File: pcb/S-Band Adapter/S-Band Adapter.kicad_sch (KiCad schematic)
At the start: 5 parts, among them J1 CT3151SP-2, J2 FTSH-107-01-L-DV-K-A, J3 ERF8-030-05.0-L-DV-TR, J4 532611071

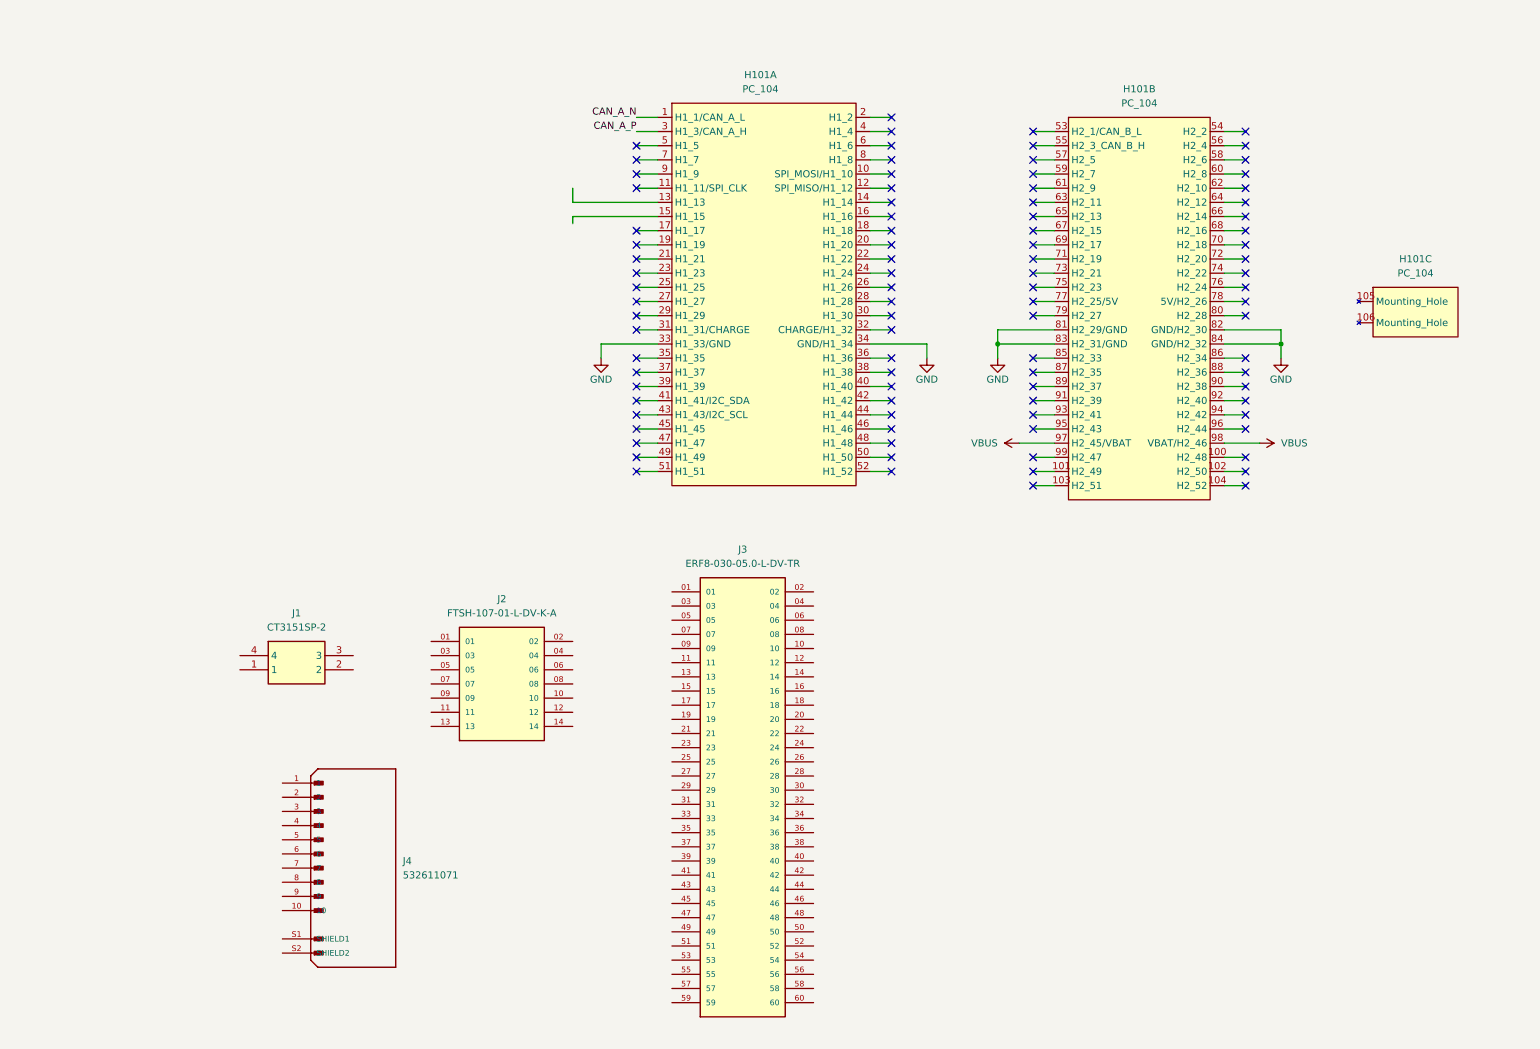
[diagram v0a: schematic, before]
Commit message: Finished PCB
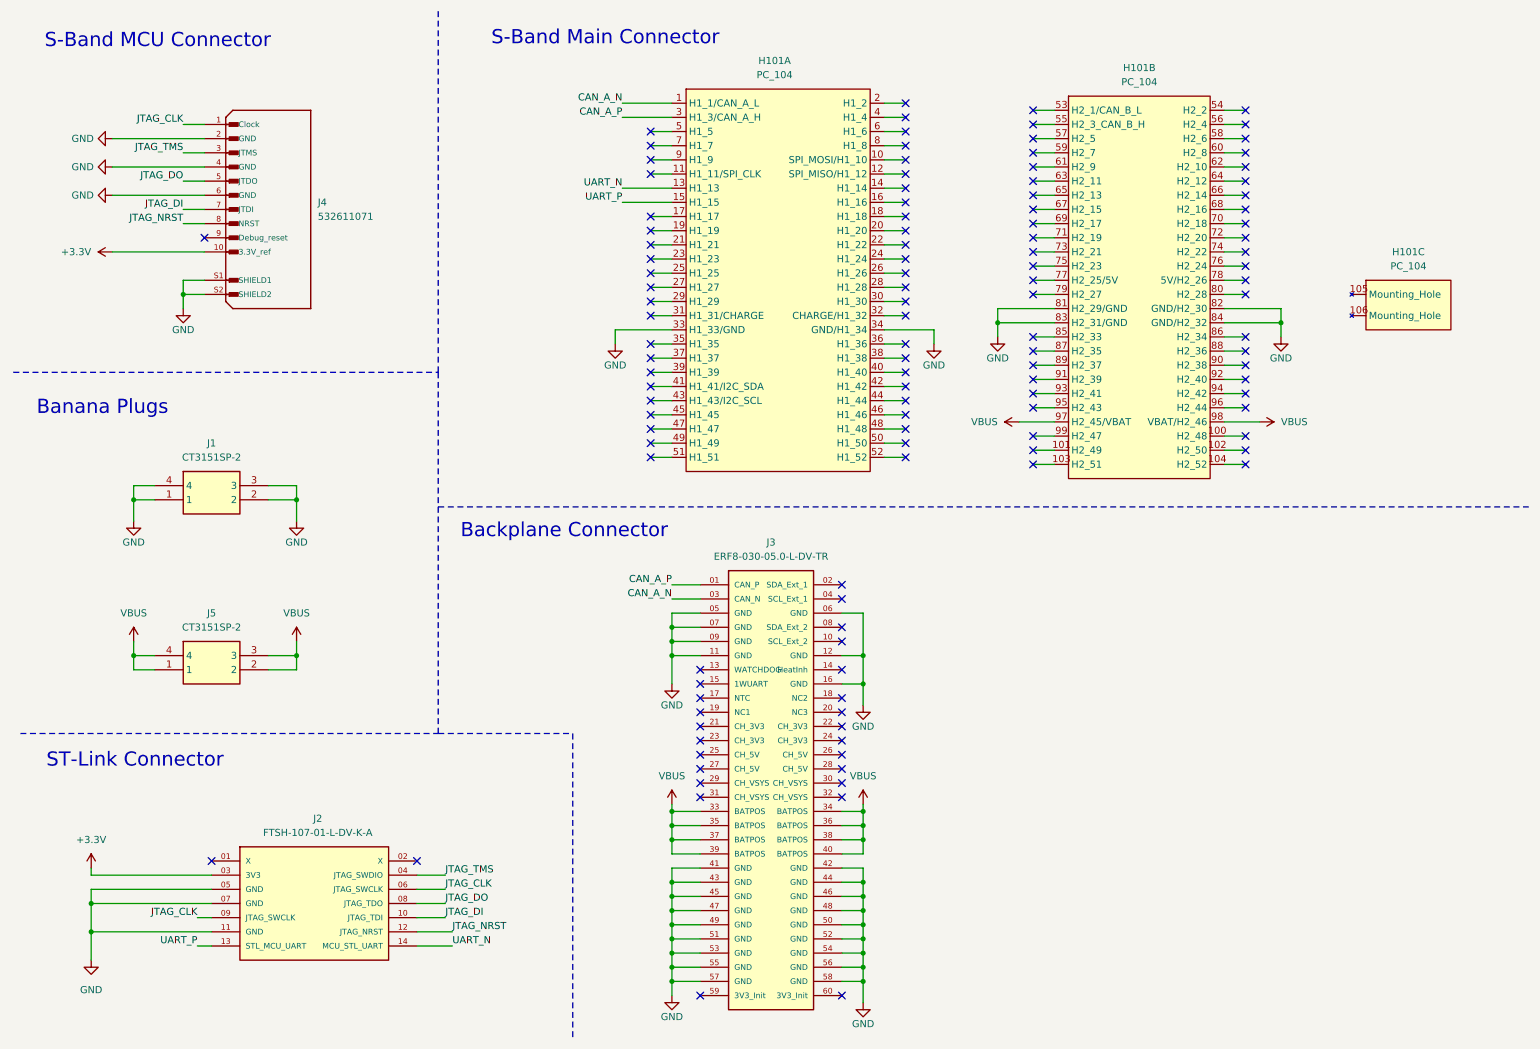
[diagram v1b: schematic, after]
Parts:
- added J5: CT3151SP-2, KiCad:CT3151SP2, symbol CT3151SP-2:CT3151SP-2
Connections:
- net CAN_A_N: now also J3.03 (CAN_N)
- net CAN_A_P: now also J3.01 (CAN_P)
- net GND: now also J1.1, J1.2, J1.3, J1.4, J2.05 (GND), J2.07 (GND), J2.11 (GND), J3.05 (GND), J3.06 (GND), J3.07 (GND), J3.09 (GND), J3.11 (GND), J3.12 (GND), J3.16 (GND), J3.41 (GND), J3.42 (GND), J3.43 (GND), J3.44 (GND), J3.45 (GND), J3.46 (GND), J3.47 (GND), J3.48 (GND), J3.49 (GND), J3.50 (GND), J3.51 (GND), J3.52 (GND), J3.53 (GND), J3.54 (GND), J3.55 (GND), J3.56 (GND), J3.57 (GND), J3.58 (GND), J4.2 (GND), J4.4 (GND), J4.6 (GND), J4.S1 (SHIELD1), J4.S2 (SHIELD2)
- net VBUS: now also J3.33 (BATPOS), J3.34 (BATPOS), J3.35 (BATPOS), J3.36 (BATPOS), J3.37 (BATPOS), J3.38 (BATPOS), J3.39 (BATPOS), J3.40 (BATPOS), J5.1, J5.2, J5.3, J5.4
- net +3.3V: now reaches J2.03 (3V3)
- net +3.3V: now also J4.10 (3.3V_ref)
- net JTAG_TMS: now reaches J2.04 (JTAG_SWDIO)
- net JTAG_TMS: now also J4.3 (JTMS)
- net JTAG_CLK: now reaches J2.06 (JTAG_SWCLK)
- net JTAG_CLK: now also J2.09 (JTAG_SWCLK), J4.1 (Clock)
- net JTAG_DO: now reaches J2.08 (JTAG_TDO)
- net JTAG_DO: now also J4.5 (JTDO)
- net JTAG_DI: now reaches J2.10 (JTAG_TDI)
- net JTAG_DI: now also J4.7 (JTDI)
- net JTAG_NRST: now reaches J2.12 (JTAG_NRST)
- net JTAG_NRST: now also J4.8 (NRST)
- net UART_P: now reaches J2.13 (STL_MCU_UART)
- net UART_P: now also H101.15 (H1_15)
- net UART_N: now reaches J2.14 (MCU_STL_UART)
- net UART_N: now also H101.13 (H1_13)
- no-connect marks 92 -> 120
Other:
- note added: "Backplane Connector"
- note added: "Banana Plugs"
- note added: "S-Band MCU Connector"
- note added: "S-Band Main Connector"
- note added: "ST-Link Connector"
- moved on the sheet: H101A, H101B, H101C, J1, J2, J3, J4
